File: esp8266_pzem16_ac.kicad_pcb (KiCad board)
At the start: 2 copper layers, 50 x 27 mm, 19 parts, among them J1 RS485, J2 PWR, J3 LED, U1 ESP-12F, U2 AMS1117-3.3

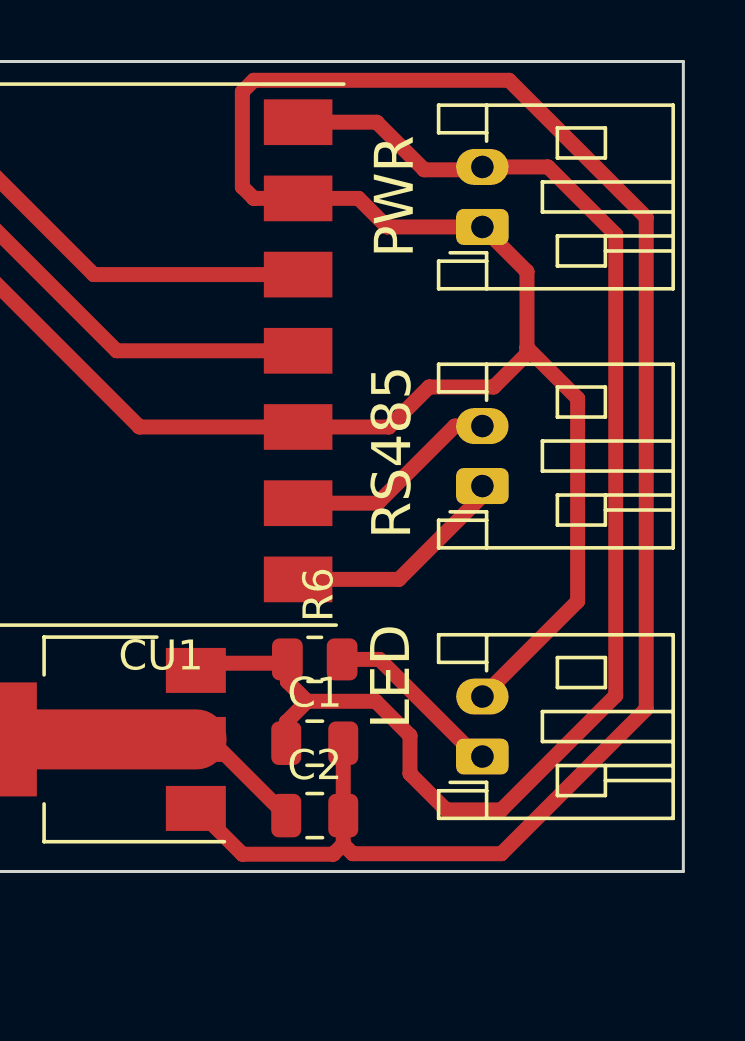
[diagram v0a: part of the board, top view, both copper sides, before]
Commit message: generated files
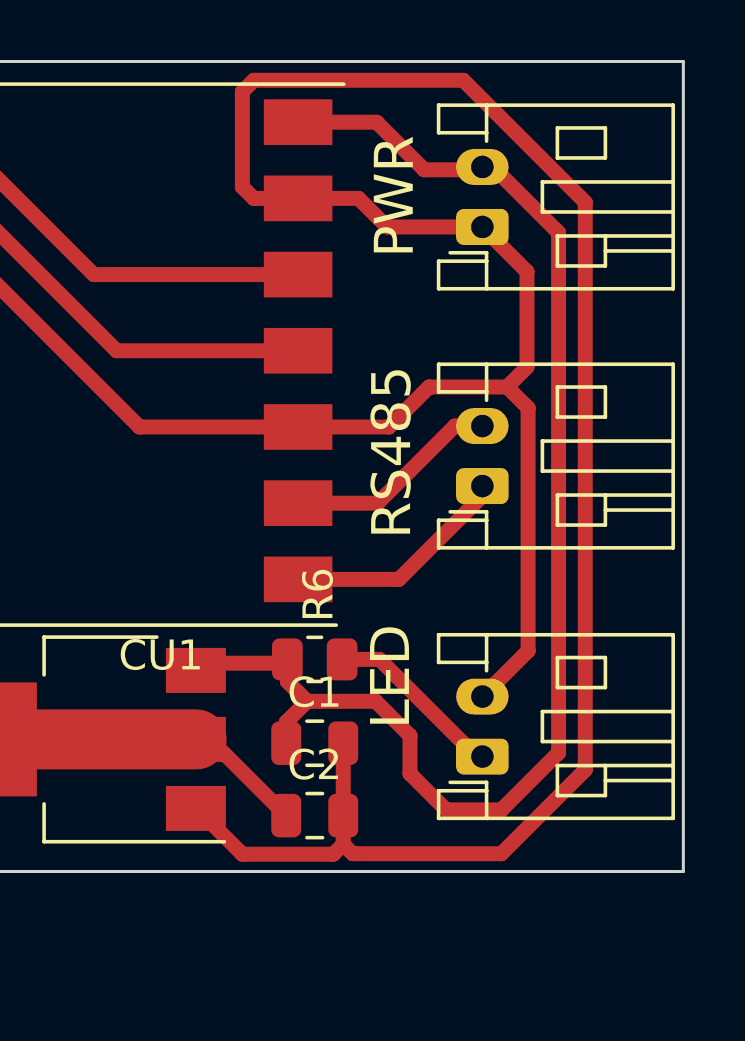
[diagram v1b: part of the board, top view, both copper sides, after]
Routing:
- net GND: track 112.3 -> 107.6 mm
- net +5V: track 48.2 -> 45.6 mm
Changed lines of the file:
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@@
   (segment (start 118.7765 57.023) (end 116.6495 57.023) (width 0.5) (layer "F.Cu") (net 1))
   (segment (start 116.6495 57.023) (end 116.332 57.3405) (width 0.5) (layer "F.Cu") (net 1))
-  (segment (start 126.746 60.7695) (end 126.746 76.1365) (width 0.5) (layer "F.Cu") (net 1))
   (segment (start 120.364 58.6105) (end 118.7765 57.023) (width 0.5) (layer "F.Cu") (net 1))
+  (segment (start 121.0945 79.9465) (end 119.888 78.74) (width 0.5) (layer "F.Cu") (net 1))
+  (segment (start 122.301 58.5155) (end 122.6505 58.5155) (width 0.5) (layer "F.Cu") (net 1))
   (segment (start 116.459 76.327) (end 115.8005 75.6685) (width 0.5) (layer "F.Cu") (net 1))
-  (segment (start 119.888 77.47) (end 118.745 76.327) (width 0.5) (layer "F.Cu") (net 1))
-  (segment (start 122.301 58.5155) (end 124.492 58.5155) (width 0.5) (layer "F.Cu") (net 1))
   (segment (start 119.888 78.74) (end 119.888 77.47) (width 0.5) (layer "F.Cu") (net 1))
+  (segment (start 122.936 79.9465) (end 121.0945 79.9465) (width 0.5) (layer "F.Cu") (net 1))
   (segment (start 115.8005 75.6685) (end 115.8005 74.93) (width 0.5) (layer "F.Cu") (net 1))
   (segment (start 115.6735 75.057) (end 113.016 75.057) (width 0.5) (layer "F.Cu") (net 1))
   (segment (start 115.8005 74.93) (end 115.6735 75.057) (width 0.5) (layer "F.Cu") (net 1))
-  (segment (start 122.936 79.9465) (end 121.0945 79.9465) (width 0.5) (layer "F.Cu") (net 1))
+  (segment (start 124.841 78.0415) (end 122.936 79.9465) (width 0.5) (layer "F.Cu") (net 1))
+  (segment (start 118.745 76.327) (end 116.459 76.327) (width 0.5) (layer "F.Cu") (net 1))
   (segment (start 113.016 75.057) (end 112.776 75.297) (width 0.5) (layer "F.Cu") (net 1))
   (segment (start 122.206 58.6105) (end 120.364 58.6105) (width 0.5) (layer "F.Cu") (net 1))
   (segment (start 122.301 58.5155) (end 122.206 58.6105) (width 0.5) (layer "F.Cu") (net 1))
-  (segment (start 118.745 76.327) (end 116.459 76.327) (width 0.5) (layer "F.Cu") (net 1))
+  (segment (start 122.6505 58.5155) (end 124.841 60.706) (width 0.5) (layer "F.Cu") (net 1))
+  (segment (start 124.841 60.706) (end 124.841 78.0415) (width 0.5) (layer "F.Cu") (net 1))
   (segment (start 115.763 77.023) (end 115.763 77.724) (width 0.5) (layer "F.Cu") (net 1))
-  (segment (start 124.492 58.5155) (end 126.746 60.7695) (width 0.5) (layer "F.Cu") (net 1))
-  (segment (start 126.746 76.1365) (end 122.936 79.9465) (width 0.5) (layer "F.Cu") (net 1))
-  (segment (start 121.0945 79.9465) (end 119.888 78.74) (width 0.5) (layer "F.Cu") (net 1))
+  (segment (start 119.888 77.47) (end 118.745 76.327) (width 0.5) (layer "F.Cu") (net 1))
   (segment (start 115.763 74.9675) (end 115.8005 74.93) (width 0.5) (layer "F.Cu") (net 1))
   (segment (start 116.459 76.327) (end 115.763 77.023) (width 0.5) (layer "F.Cu") (net 1))
@@
   (segment (start 117.3305 81.4245) (end 114.3035 81.4245) (width 0.5) (layer "F.Cu") (net 2))
   (segment (start 116.159 59.7075) (end 116.332 59.8805) (width 0.5) (layer "F.Cu") (net 2))
-  (segment (start 120.523 65.8495) (end 122.682 65.8495) (width 0.5) (layer "F.Cu") (net 2))
+  (segment (start 119.1895 67.183) (end 120.523 65.8495) (width 0.5) (layer "F.Cu") (net 2))
   (segment (start 122.301 60.5155) (end 119.126 60.5155) (width 0.5) (layer "F.Cu") (net 2))
-  (segment (start 125.476 72.9935) (end 122.301 76.1685) (width 0.5) (layer "F.Cu") (net 2))
+  (segment (start 123.825 74.6445) (end 122.301 76.1685) (width 0.5) (layer "F.Cu") (net 2))
   (segment (start 119.126 60.5155) (end 118.1735 59.563) (width 0.5) (layer "F.Cu") (net 2))
   (segment (start 117.663 81.092) (end 117.3305 81.4245) (width 0.5) (layer "F.Cu") (net 2))
-  (segment (start 123.788 64.7435) (end 123.788 64.5425) (width 0.5) (layer "F.Cu") (net 2))
-  (segment (start 114.681 55.626) (end 123.19 55.626) (width 0.5) (layer "F.Cu") (net 2))
-  (segment (start 119.1895 67.183) (end 120.523 65.8495) (width 0.5) (layer "F.Cu") (net 2))
+  (segment (start 123.1265 65.8495) (end 123.788 65.188) (width 0.5) (layer "F.Cu") (net 2))
+  (segment (start 114.3 56.007) (end 114.681 55.626) (width 0.5) (layer "F.Cu") (net 2))
+  (segment (start 123.825 66.548) (end 123.825 74.6445) (width 0.5) (layer "F.Cu") (net 2))
+  (segment (start 114.3035 81.4245) (end 112.776 79.897) (width 0.5) (layer "F.Cu") (net 2))
+  (segment (start 114.681 55.626) (end 121.666 55.626) (width 0.5) (layer "F.Cu") (net 2))
+  (segment (start 101.139 58.166) (end 101.94 58.967) (width 0.5) (layer "F.Cu") (net 2))
+  (segment (start 122.936 81.407) (end 117.978 81.407) (width 0.5) (layer "F.Cu") (net 2))
+  (segment (start 120.523 65.8495) (end 123.1265 65.8495) (width 0.5) (layer "F.Cu") (net 2))
+  (segment (start 101.94 58.967) (end 101.94 60.98) (width 0.5) (layer "F.Cu") (net 2))
+  (segment (start 123.1265 65.8495) (end 123.825 66.548) (width 0.5) (layer "F.Cu") (net 2))
+  (segment (start 117.663 80.137) (end 117.663 81.092) (width 0.5) (layer "F.Cu") (net 2))
   (segment (start 116.159 67.183) (end 119.1895 67.183) (width 0.5) (layer "F.Cu") (net 2))
-  (segment (start 114.3035 81.4245) (end 112.776 79.897) (width 0.5) (layer "F.Cu") (net 2))
-  (segment (start 101.139 58.166) (end 101.94 58.967) (width 0.5) (layer "F.Cu") (net 2))
-  (segment (start 127.762 76.581) (end 122.936 81.407) (width 0.5) (layer "F.Cu") (net 2))
-  (segment (start 101.94 58.967) (end 101.94 60.98) (width 0.5) (layer "F.Cu") (net 2))
-  (segment (start 117.663 80.137) (end 117.663 81.092) (width 0.5) (layer "F.Cu") (net 2))
   (segment (start 118.1735 59.563) (end 116.159 59.563) (width 0.5) (layer "F.Cu") (net 2))
+  (segment (start 123.788 65.188) (end 123.788 62.0025) (width 0.5) (layer "F.Cu") (net 2))
+  (segment (start 114.3 59.182) (end 114.3 56.007) (width 0.5) (layer "F.Cu") (net 2))
+  (segment (start 123.788 62.0025) (end 122.301 60.5155) (width 0.5) (layer "F.Cu") (net 2))
+  (segment (start 117.663 80.137) (end 117.663 77.724) (width 0.5) (layer "F.Cu") (net 2))
+  (segment (start 121.666 55.626) (end 125.73 59.69) (width 0.5) (layer "F.Cu") (net 2))
   (segment (start 114.681 59.563) (end 114.3 59.182) (width 0.5) (layer "F.Cu") (net 2))
-  (segment (start 122.936 81.407) (end 117.978 81.407) (width 0.5) (layer "F.Cu") (net 2))
-  (segment (start 117.663 80.137) (end 117.663 77.724) (width 0.5) (layer "F.Cu") (net 2))
-  (segment (start 114.3 56.007) (end 114.681 55.626) (width 0.5) (layer "F.Cu") (net 2))
-  (segment (start 125.476 66.2305) (end 125.476 72.9935) (width 0.5) (layer "F.Cu") (net 2))
-  (segment (start 122.682 65.8495) (end 123.788 64.7435) (width 0.5) (layer "F.Cu") (net 2))
-  (segment (start 123.19 55.626) (end 127.762 60.198) (width 0.5) (layer "F.Cu") (net 2))
-  (segment (start 123.788 64.5425) (end 125.476 66.2305) (width 0.5) (layer "F.Cu") (net 2))
+  (segment (start 117.978 81.407) (end 117.663 81.092) (width 0.5) (layer "F.Cu") (net 2))
+  (segment (start 125.73 59.69) (end 125.73 78.613) (width 0.5) (layer "F.Cu") (net 2))
+  (segment (start 125.73 78.613) (end 122.936 81.407) (width 0.5) (layer "F.Cu") (net 2))
   (segment (start 116.159 67.183) (end 110.871 67.183) (width 0.5) (layer "F.Cu") (net 2))
-  (segment (start 127.762 60.198) (end 127.762 76.581) (width 0.5) (layer "F.Cu") (net 2))
   (segment (start 116.159 59.563) (end 114.681 59.563) (width 0.5) (layer "F.Cu") (net 2))
   (segment (start 116.159 59.563) (end 116.159 59.7075) (width 0.5) (layer "F.Cu") (net 2))
-  (segment (start 117.978 81.407) (end 117.663 81.092) (width 0.5) (layer "F.Cu") (net 2))
   (segment (start 104.668 60.98) (end 101.94 60.98) (width 0.5) (layer "F.Cu") (net 2))
-  (segment (start 114.3 59.182) (end 114.3 56.007) (width 0.5) (layer "F.Cu") (net 2))
-  (segment (start 123.788 62.0025) (end 123.788 64.5425) (width 0.5) (layer "F.Cu") (net 2))
-  (segment (start 122.301 60.5155) (end 123.788 62.0025) (width 0.5) (layer "F.Cu") (net 2))
   (segment (start 106.476 77.597) (end 103.357 77.597) (width 0.5) (layer "F.Cu") (net 3))
   (segment (start 93.8765 79.4785) (end 93.8765 78.867) (width 0.5) (layer "F.Cu") (net 3))
